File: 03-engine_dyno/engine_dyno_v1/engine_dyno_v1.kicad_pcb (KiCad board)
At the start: 4 copper layers, 101.3 x 69 mm, 91 parts, among them J1 Screw_Terminal_01x02, J4 Screw_Terminal_01x05, J5 Screw_Terminal_01x03, J6 Screw_Terminal_01x05, J7 Screw_Terminal_01x03, P1 J1B1211CCD, Q1 PMOS, U1 LMR51430XDDCR, U10 INA827AIDGKR, U11 74LVC1G17, U12 AD630ARZ, U13 ADS1120IPWR, U14 OPA192IDBVR, U15 OPA192IDBVR, U16 74LVC1G17, U2 TVS1800DRV, U3 TPS2115APWR, U4 TPS60403DBVRG4, U5 AD5689RBRUZ, U6 Teensy4.1, U7 INA827AIDGKR, U8 AD630ARZ, U9 ADS1120IPWR

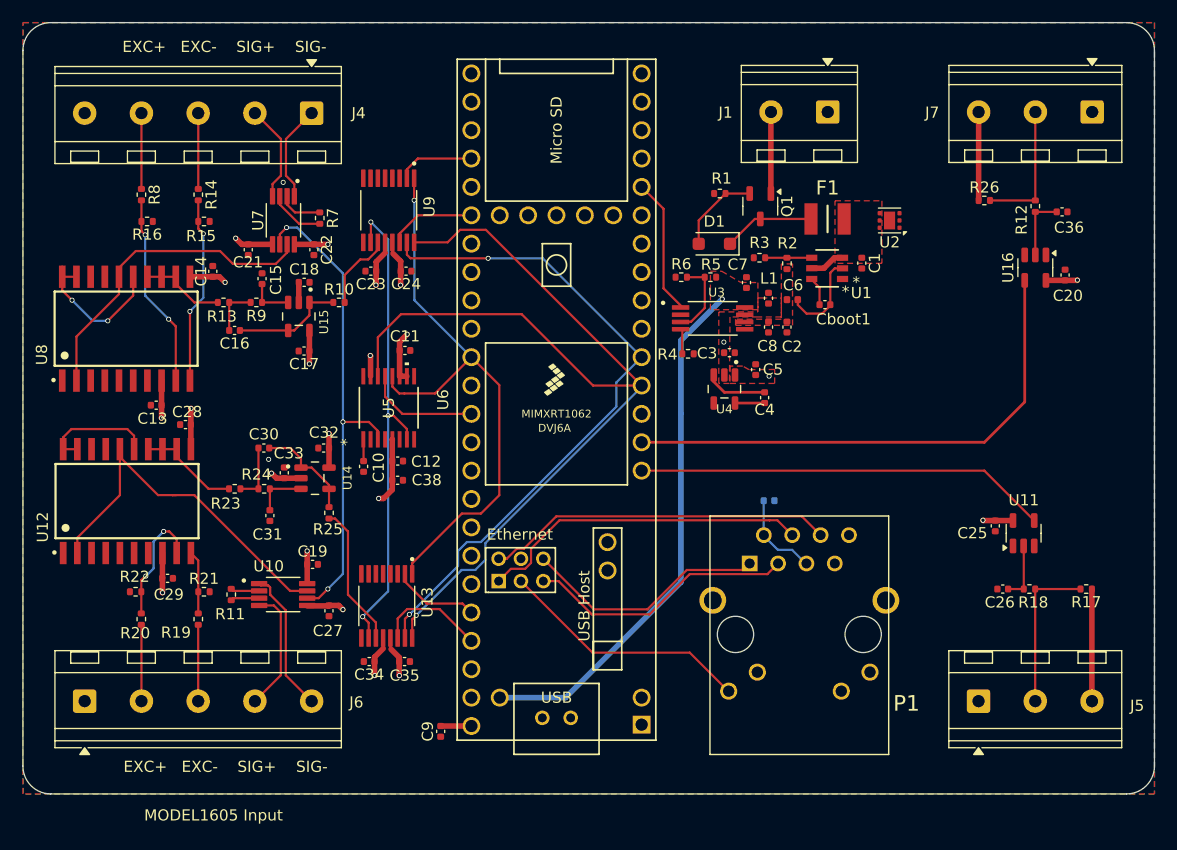
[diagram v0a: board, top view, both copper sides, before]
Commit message: im aboutta release
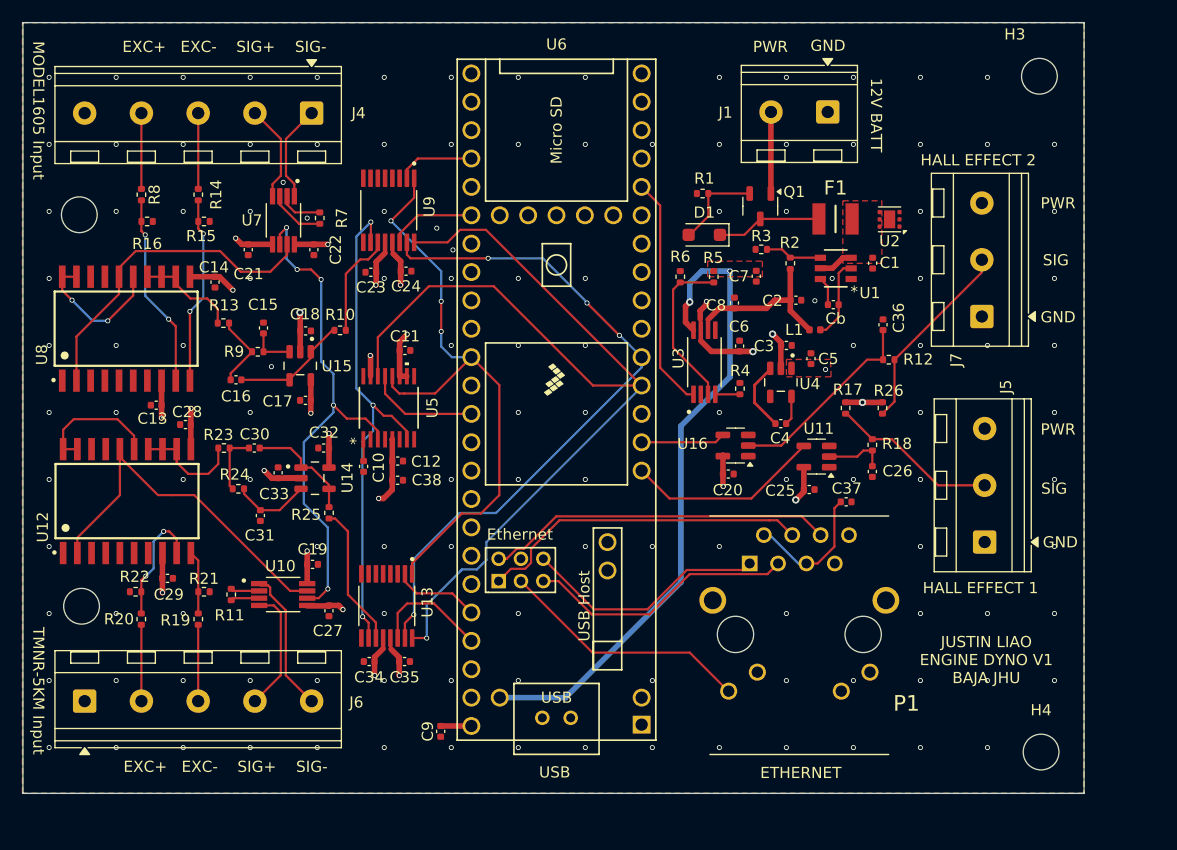
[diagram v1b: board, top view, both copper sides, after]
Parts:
- added H1: MountingHole, MountingHole:MountingHole_3.2mm_M3_DIN965, F.Cu at (108.5, 73.0)
- added H2: MountingHole, MountingHole:MountingHole_3.2mm_M3_DIN965, F.Cu at (108.7, 108.0)
- added H3: MountingHole, MountingHole:MountingHole_3.2mm_M3_DIN965, F.Cu at (194.4, 60.6)
- added H4: MountingHole, MountingHole:MountingHole_3.2mm_M3_DIN965, F.Cu at (194.6, 121.1)
- C37: moved to F.Cu
- moved C20 35.0 mm to (166.6, 96.2), turned to 0 degrees
- moved U16 31.2 mm to (167.2, 93.7), turned to 180 degrees
- moved R17 27.0 mm to (177.1, 90.3), turned to -90 degrees
- moved J7 20.8 mm to (189.3, 82.1), turned to 90 degrees
- moved R26 20.7 mm to (180.4, 90.3), turned to -90 degrees
- moved U11 19.8 mm to (174.5, 94.7), turned to 180 degrees
- moved R18 19.1 mm to (179.5, 93.6), turned to -90 degrees
- moved R12 19.0 mm to (181.0, 86.0), turned to 180 degrees
- moved C36 19.0 mm to (180.4, 82.8), turned to -90 degrees
- moved C25 17.0 mm to (173.8, 97.6), turned to 0 degrees
- moved C26 15.7 mm to (179.5, 96.0), turned to 90 degrees
- moved J5 14.3 mm to (189.6, 102.3), turned to 90 degrees
- moved C37 6.90 mm to (177.2, 98.7)
- moved R4 5.59 mm to (167.6, 88.6), turned to 90 degrees
- moved C3 5.14 mm to (171.8, 84.7)
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- renumbered Cboot1 to Cb
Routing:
- net /Hall1/HALL: track 46.7 -> 7.54 mm
- net /Hall2/HALL: track 37.0 -> 17.5 mm
- net /power/+5V_BUCK: track 0.00 -> 15.2 mm
- net Net-(C36-Pad2): track 5.77 -> 17.9 mm
- net /MCU/+5V_USB: track 47.4 -> 58.9 mm, vias 1 -> 2
- net /MCU/A16: track 12.3 -> 20.8 mm
- net Net-(U3-D1): track 6.87 -> 14.6 mm
- net /Hall1/SIG: track 11.9 -> 17.5 mm
- net Net-(P1-RCT): track 7.99 -> 12.2 mm
- net -5V: track 18.4 -> 22.4 mm, vias 6 -> 7
- net /MCU/MOSI: track 89.0 -> 92.1 mm
- net /MCU/SCK: track 52.4 -> 55.2 mm, vias 1 -> 3
- net /Model1605/BIAS_REF: track 43.8 -> 46.4 mm, vias 3 -> 5
- net /Model1605/OPA192_OUT: track 7.02 -> 9.48 mm
- net Net-(C16-Pad2): track 4.36 -> 6.73 mm
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- removed copper zone on F.Cu, net +5V
- removed copper zone on F.Cu, net /power/+5V_BUCK
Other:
- board size 101.3 x 69 mm -> 95 x 69 mm
- board text added: "12V BATT"
- board text added: "ETHERNET"
- board text added: "GND"
- board text added: "HALL EFFECT 1"
- board text added: "HALL EFFECT 2"
- board text added: "JUSTIN LIAO ENGINE DYNO V1 BAJA JHU"
- board text added: "PWR"
- board text added: "SIG"
- board text added: "TMNR-5KM Input"
- board text added: "USB"
